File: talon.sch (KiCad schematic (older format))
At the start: 10 parts, among them U1 LCMXO2-256HC-4SG32C, U2 AZ1117-3.3V

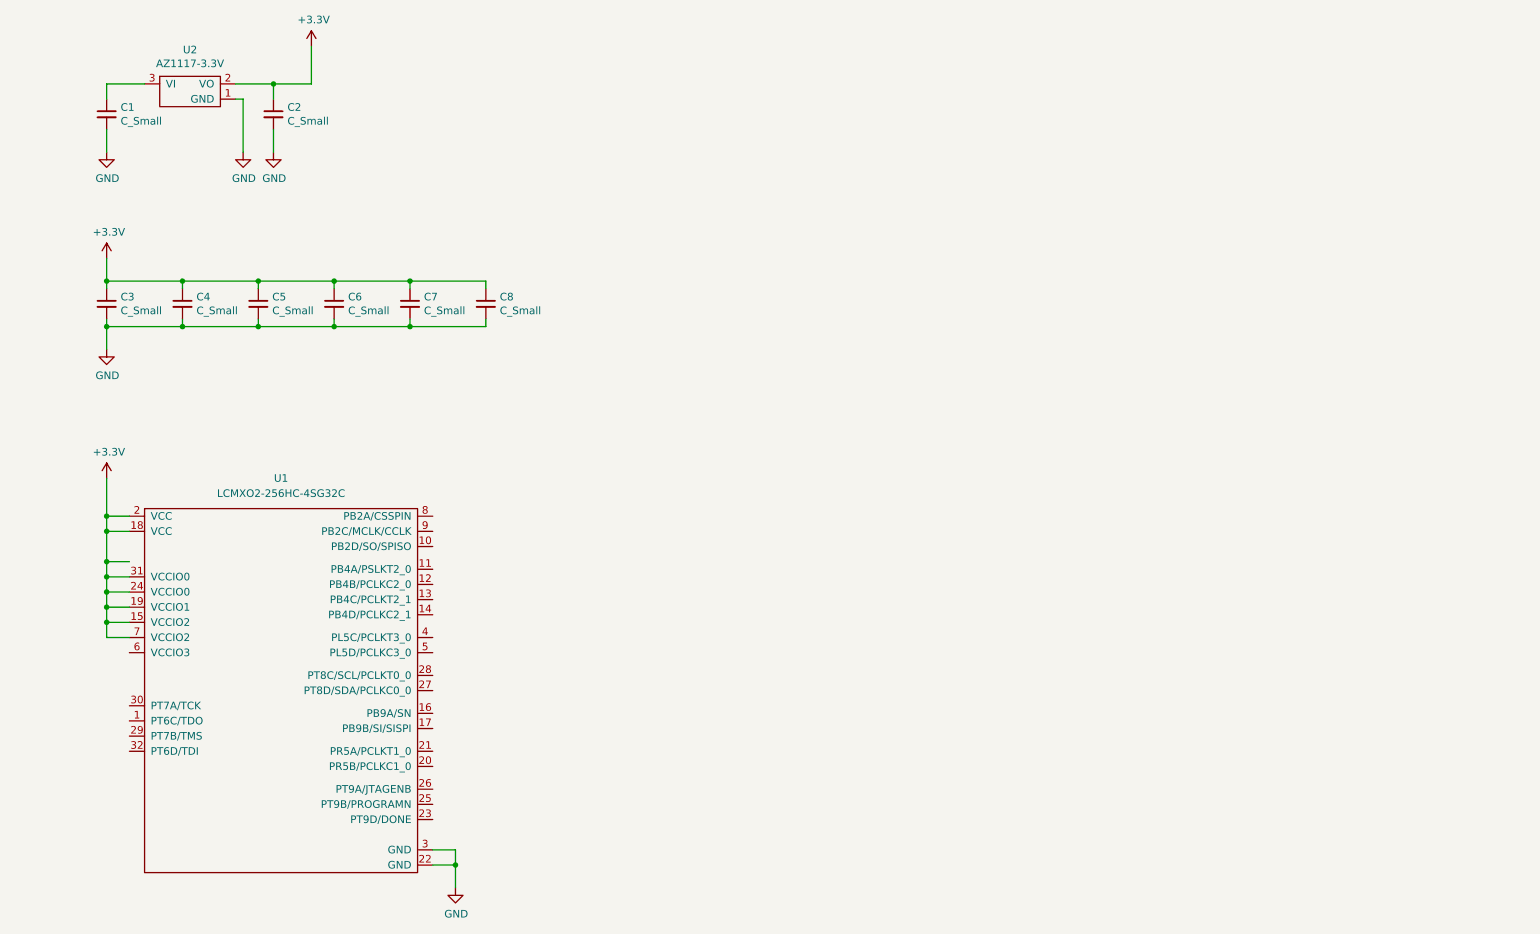
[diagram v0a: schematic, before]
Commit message: FPGA wired and ready
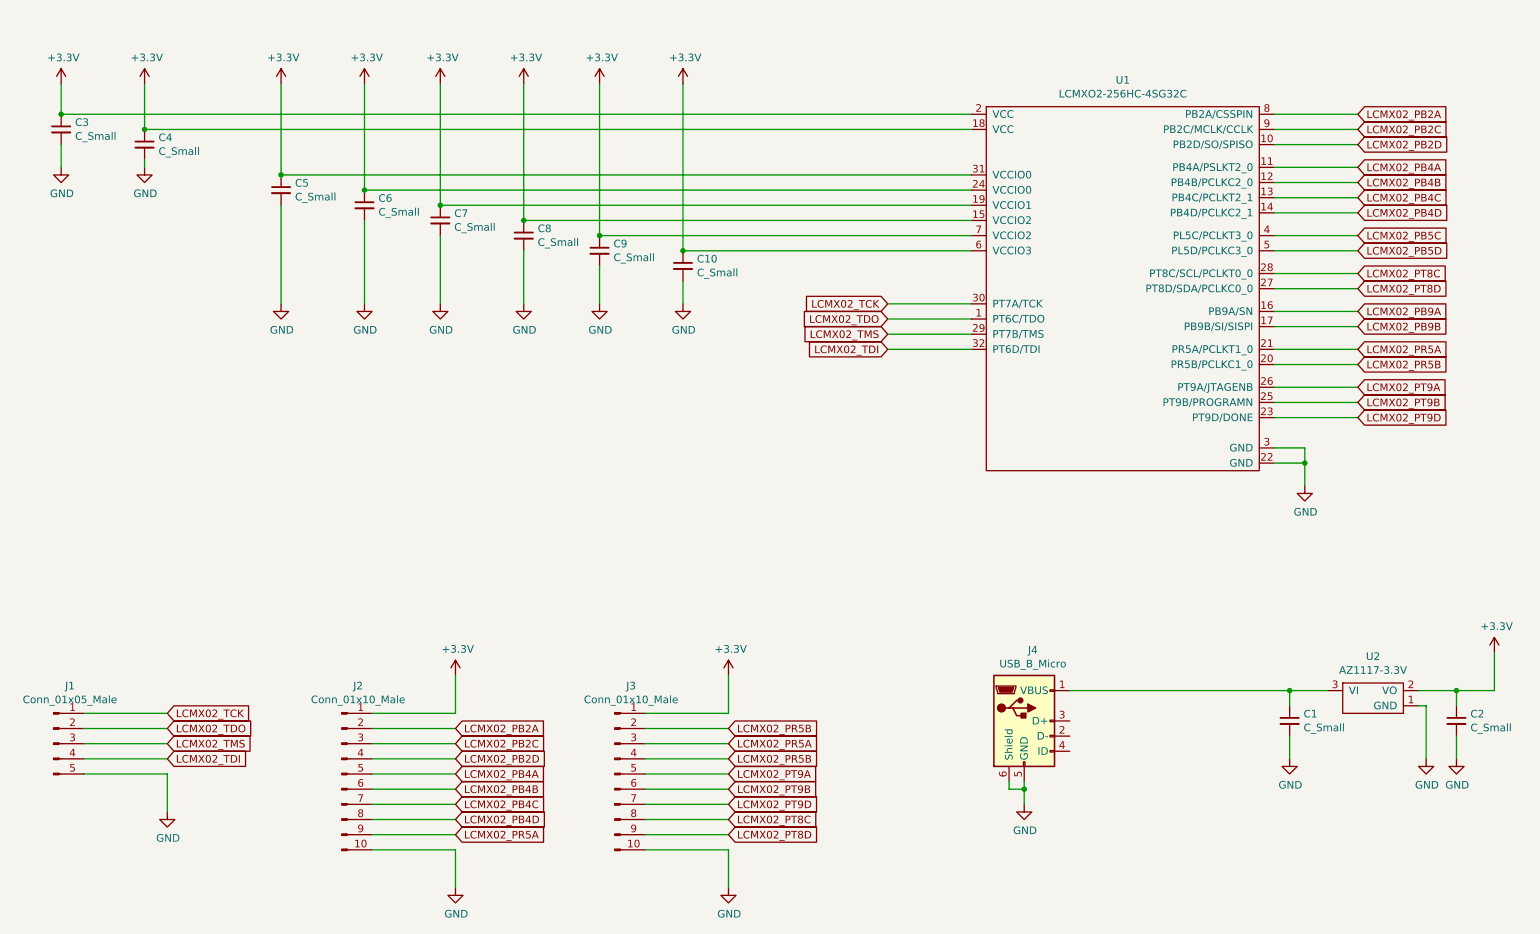
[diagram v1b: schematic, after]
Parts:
- removed C3, C4: C_Small, symbol Device:C_Small
- added C10, C7, C8, C9: C_Small, symbol Device:C_Small
- added J1: Conn_01x05_Male, symbol Connector:Conn_01x05_Male
- added J2, J3: Conn_01x10_Male, symbol Connector:Conn_01x10_Male
- added J4: USB_B_Micro, symbol Connector:USB_B_Micro
- renumbered C7 to C3, C8 to C4
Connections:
- net +3V3: now also U1.6 (VCCIO3), C10.1, C7.1, C8.1, C9.1, J2.1 (Pin_1), J3.1 (Pin_1)
- net GND: now also C10.2, C7.2, C8.2, C9.2, J1.5 (Pin_5), J2.10 (Pin_10), J3.10 (Pin_10), J4.5 (GND), J4.6 (Shield)
- net at C1.1, U2.3 (VI): now also J4.1 (VBUS)
- net LCMX02_TDO: now reaches U1.1 (PT6C/TDO)
- net LCMX02_TDO: now also J1.2 (Pin_2)
- net LCMX02_PB2D: now reaches U1.10 (PB2D/SO/SPISO)
- net LCMX02_PB2D: now also J2.4 (Pin_4)
- net LCMX02_PB4A: now reaches U1.11 (PB4A/PSLKT2_0)
- net LCMX02_PB4A: now also J2.5 (Pin_5)
- net LCMX02_PB4B: now reaches U1.12 (PB4B/PCLKC2_0)
- net LCMX02_PB4B: now also J2.6 (Pin_6)
- net LCMX02_PB4C: now reaches U1.13 (PB4C/PCLKT2_1)
- net LCMX02_PB4C: now also J2.7 (Pin_7)
- net LCMX02_PB4D: now reaches U1.14 (PB4D/PCLKC2_1)
- net LCMX02_PB4D: now also J2.8 (Pin_8)
- net LCMX02_PB9A: now reaches U1.16 (PB9A/SN)
- net LCMX02_PB9B: now reaches U1.17 (PB9B/SI/SISPI)
- net LCMX02_PR5B: now reaches U1.20 (PR5B/PCLKC1_0)
- net LCMX02_PR5B: now also J3.2 (Pin_2), J3.4 (Pin_4)
- net LCMX02_PR5A: now reaches U1.21 (PR5A/PCLKT1_0)
- net LCMX02_PR5A: now also J2.9 (Pin_9), J3.3 (Pin_3)
- net LCMX02_PT9D: now reaches U1.23 (PT9D/DONE)
- net LCMX02_PT9D: now also J3.7 (Pin_7)
- net LCMX02_PT9B: now reaches U1.25 (PT9B/PROGRAMN)
- net LCMX02_PT9B: now also J3.6 (Pin_6)
- net LCMX02_PT9A: now reaches U1.26 (PT9A/JTAGENB)
- net LCMX02_PT9A: now also J3.5 (Pin_5)
- net LCMX02_PT8D: now reaches U1.27 (PT8D/SDA/PCLKC0_0)
- net LCMX02_PT8D: now also J3.9 (Pin_9)
- net LCMX02_PT8C: now reaches U1.28 (PT8C/SCL/PCLKT0_0)
- net LCMX02_PT8C: now also J3.8 (Pin_8)
- net LCMX02_TMS: now reaches U1.29 (PT7B/TMS)
- net LCMX02_TMS: now also J1.3 (Pin_3)
- net LCMX02_TCK: now reaches U1.30 (PT7A/TCK)
- net LCMX02_TCK: now also J1.1 (Pin_1)
- net LCMX02_TDI: now reaches U1.32 (PT6D/TDI)
- net LCMX02_TDI: now also J1.4 (Pin_4)
- net LCMX02_PB5C: now reaches U1.4 (PL5C/PCLKT3_0)
- net LCMX02_PB5D: now reaches U1.5 (PL5D/PCLKC3_0)
- net LCMX02_PB2A: now reaches U1.8 (PB2A/CSSPIN)
- net LCMX02_PB2A: now also J2.2 (Pin_2)
- net LCMX02_PB2C: now reaches U1.9 (PB2C/MCLK/CCLK)
- net LCMX02_PB2C: now also J2.3 (Pin_3)
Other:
- moved on the sheet: C1, C2, C3, C4, U2
